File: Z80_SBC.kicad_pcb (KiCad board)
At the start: 2 copper layers, 100 x 100 mm, 11 parts, among them U1 Z80CPU, U2 HM62256BLP, U3 27C64, U4 74HCT04, U5 74LS139, U6 MC68A50, Y1 1.8432MHz

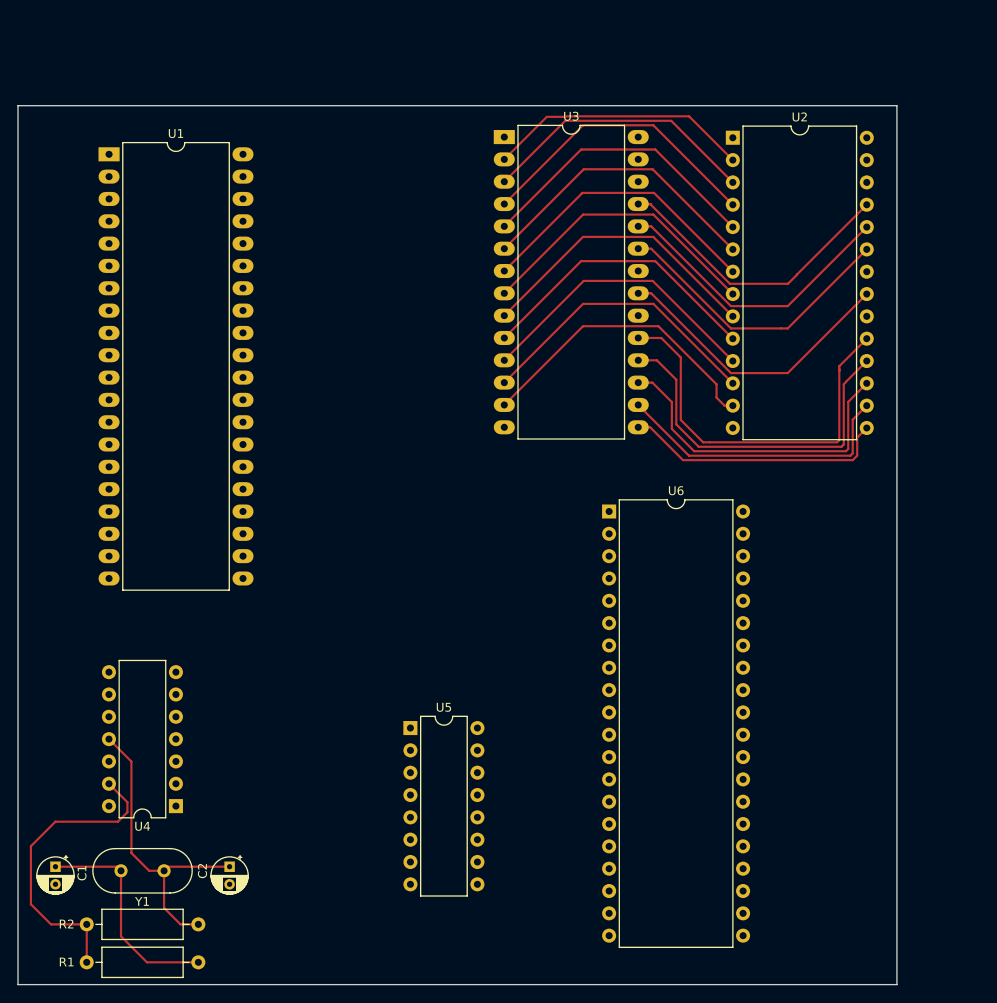
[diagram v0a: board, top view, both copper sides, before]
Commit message: poor route
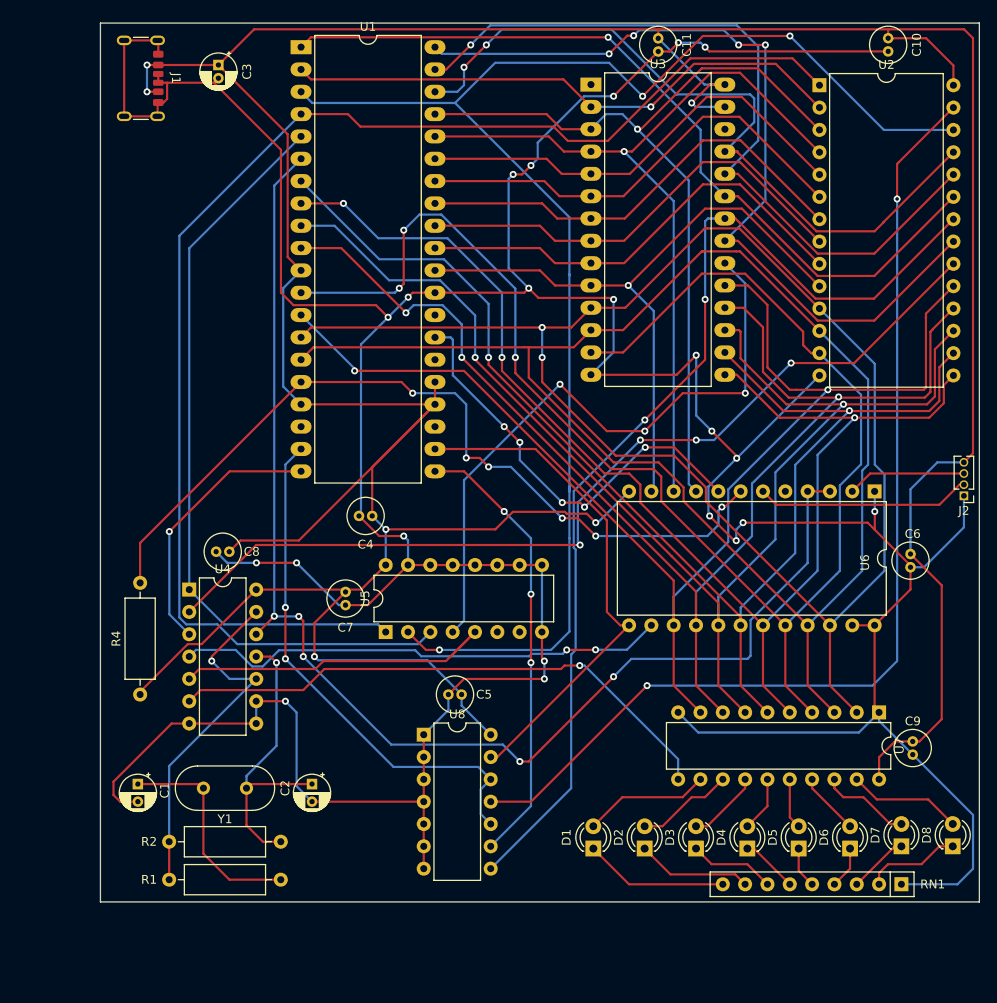
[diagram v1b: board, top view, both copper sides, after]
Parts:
- added C10: 0.1uF, Capacitor_THT:C_Radial_D4.0mm_H5.0mm_P1.50mm, F.Cu at (188.0, 39.1)
- added C11: 0.1uF, Capacitor_THT:C_Radial_D4.0mm_H5.0mm_P1.50mm, F.Cu at (161.8, 39.1)
- added C3: 100uF, Capacitor_THT:CP_Radial_D4.0mm_P1.50mm, F.Cu at (111.8, 42.2)
- added C4: 0.1uF, Capacitor_THT:C_Radial_D4.0mm_H5.0mm_P1.50mm, F.Cu at (129.3, 93.5)
- added C5: 0.1uF, Capacitor_THT:C_Radial_D4.0mm_H5.0mm_P1.50mm, F.Cu at (139.4, 113.8)
- added C6: 0.1uF, Capacitor_THT:C_Radial_D4.0mm_H5.0mm_P1.50mm, F.Cu at (190.5, 97.8)
- added C7: 0.1uF, Capacitor_THT:C_Radial_D4.0mm_H5.0mm_P1.50mm, F.Cu at (126.2, 102.1)
- added C8: 0.1uF, Capacitor_THT:C_Radial_D4.0mm_H5.0mm_P1.50mm, F.Cu at (113.0, 97.5)
- added C9: 0.1uF, Capacitor_THT:C_Radial_D4.0mm_H5.0mm_P1.50mm, F.Cu at (190.8, 119.1)
- added D1: LED, LED_THT:LED_D3.0mm, F.Cu at (154.4, 131.3)
- added D2: LED, LED_THT:LED_D3.0mm, F.Cu at (160.3, 131.3)
- added D3: LED, LED_THT:LED_D3.0mm, F.Cu at (166.1, 131.3)
- added D4: LED, LED_THT:LED_D3.0mm, F.Cu at (171.9, 131.3)
- added D5: LED, LED_THT:LED_D3.0mm, F.Cu at (177.8, 131.3)
- added D6: LED, LED_THT:LED_D3.0mm, F.Cu at (183.6, 131.3)
- added D7: LED, LED_THT:LED_D3.0mm, F.Cu at (189.5, 131.1)
- added D8: LED, LED_THT:LED_D3.0mm, F.Cu at (195.3, 131.1)
- added J1: USB_C_Receptacle_PowerOnly_6P, Connector_USB:USB_C_Receptacle_GCT_USB4125-xx-x_6P_TopMnt_Horizontal, F.Cu at (101.8, 43.7)
- added J2: Conn_01x04_Pin, Connector_PinHeader_1.27mm:PinHeader_1x04_P1.27mm_Vertical, F.Cu at (196.6, 91.2)
- added R4: 3k3, Resistor_THT:R_Axial_DIN0309_L9.0mm_D3.2mm_P12.70mm_Horizontal, F.Cu at (102.8, 113.8)
- added RN1: R_Network08, Resistor_THT:R_Array_SIP9, F.Cu at (189.5, 135.4)
- added U7: 74LS573, Package_DIP:DIP-20_W7.62mm, F.Cu at (186.9, 115.8)
- added U8: 74LS32, Package_DIP:DIP-14_W7.62mm, F.Cu at (135.1, 118.4)
- U6: footprint Package_DIP:DIP-40_W15.24mm -> Package_DIP:DIP-24_W15.24mm
- moved U6 30.3 mm to (186.4, 90.7), turned to -90 degrees
- moved U1 25.0 mm to (121.2, 40.1)
- moved U4 24.7 mm to (108.4, 101.8), turned to 0 degrees
- moved C1 13.3 mm to (102.6, 124.0)
- moved C2 13.3 mm to (122.4, 124.0)
- moved R1 13.3 mm to (106.2, 134.9)
- moved R2 13.3 mm to (118.9, 130.5)
- moved Y1 13.3 mm to (115.0, 124.4)
- moved U3 11.5 mm to (154.1, 44.4)
- moved U2 11.5 mm to (180.1, 44.5)
- moved U5 11.3 mm to (130.8, 106.7), turned to 90 degrees
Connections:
- U1 pad 11: unconnected-(U1-VCC-Pad11) -> 5V
- U1 pad 16: unconnected-(U1-~{INT}-Pad16) -> ~{INT}
- U1 pad 17: unconnected-(U1-~{NMI}-Pad17) -> 5V
- U1 pad 19: unconnected-(U1-~{MREQ}-Pad19) -> ~{MREQ}
- U1 pad 20: unconnected-(U1-~{IORQ}-Pad20) -> ~{I/O}
- U1 pad 24: unconnected-(U1-~{WAIT}-Pad24) -> 5V
- U1 pad 25: unconnected-(U1-~{BUSRQ}-Pad25) -> 5V
- U1 pad 27: unconnected-(U1-~{M1}-Pad27) -> ~{M1}
- U1 pad 30: /Address0 -> A0
- U1 pad 36: /Address6 -> A6
- U1 pad 37: /Address7 -> A7
- U2 pad 10: /Address0 -> A0
- U2 pad 22: ~{RD} -> ~{MEMRD}
- U2 pad 27: ~{WR} -> ~{MEMWR}
- U2 pad 28: unconnected-(U2-VCC-Pad28) -> 5V
- U2 pad 3: /Address7 -> A7
- U2 pad 4: /Address6 -> A6
- U3 pad 10: /Address0 -> A0
- U3 pad 22: ~{RD} -> ~{MEMRD}
- U3 pad 27: unconnected-(U3-~{WE}-Pad27) -> 5V
- U3 pad 28: unconnected-(U3-VCC-Pad28) -> 5V
- U3 pad 3: /Address7 -> A7
- U3 pad 4: /Address6 -> A6
- U4 pad 14: Net-(U4G-VCC) -> 5V
- U4 pad 3: GND -> ~{I/O}
- U4 pad 4: GND -> Net-(U6-E)
- U4 pad 5: GND -> Net-(U5A-O1)
- U4 pad 6: GND -> Net-(U7-Load)
- U5 pad 16: Net-(U4G-VCC) -> 5V
- U5 pad 5: unconnected-(U5A-O1-Pad5) -> Net-(U5A-O1)
- U6 pad 10: unconnected-(U6-CS1-Pad10) -> A6
- U6 pad 11: unconnected-(U6-RS-Pad11) -> A0
- U6 pad 12: unconnected-(U6-VCC-Pad12) -> 5V
- U6 pad 13: unconnected-(U6-R/~{W}-Pad13) -> ~{WR}
- U6 pad 14: unconnected-(U6-E-Pad14) -> Net-(U6-E)
- U6 pad 2: unconnected-(U6-Rx_Data-Pad2) -> RX
- U6 pad 23: unconnected-(U6-~{DCD}-Pad23) -> GND
- U6 pad 24: unconnected-(U6-~{CTS}-Pad24) -> GND
- U6 pad 3: unconnected-(U6-Rx_CLK-Pad3) -> CLK
- U6 pad 4: unconnected-(U6-Tx_CLK-Pad4) -> CLK
- U6 pad 6: unconnected-(U6-Tx_Data-Pad6) -> TX
- U6 pad 7: unconnected-(U6-~{IRQ}-Pad7) -> ~{INT}
- U6 pad 8: unconnected-(U6-CS0-Pad8) -> ~{M1}
- U6 pad 9: unconnected-(U6-CS2-Pad9) -> A7
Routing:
- net GND: track 0.00 -> 516.5 mm, vias 0 -> 22
- net 5V: track 0.00 -> 439.3 mm, vias 0 -> 6
- net A13: track 0.00 -> 171.7 mm, vias 0 -> 3
- net A14: track 0.00 -> 158.8 mm
- net CLK: track 0.00 -> 148.6 mm, vias 0 -> 5
- net /Data0: track 33.5 -> 172.1 mm, vias 0 -> 2
- net /Data2: track 34.3 -> 171.4 mm, vias 0 -> 3
- net /Data1: track 33.5 -> 165.4 mm
- net ~{MEMRD}: track 0.00 -> 119.8 mm, vias 0 -> 2
- net /Data3: track 30.6 -> 149.4 mm, vias 0 -> 3
- net ~{MEMWR}: track 0.00 -> 118.5 mm, vias 0 -> 2
- net /Data4: track 33.0 -> 150.0 mm, vias 0 -> 2
- net /Data5: track 37.4 -> 150.9 mm, vias 0 -> 2
- net /Data6: track 41.1 -> 153.2 mm, vias 0 -> 3
- net Net-(U2-~{CS}): track 0.00 -> 106.7 mm, vias 0 -> 4
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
